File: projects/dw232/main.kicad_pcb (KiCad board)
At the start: 4 copper layers, 27 parts, among them P101 CONN_01X07, Q501 MMBT3904, Q502 MMBT3904, U501 LM741, U502 LM741, U503 2DW232

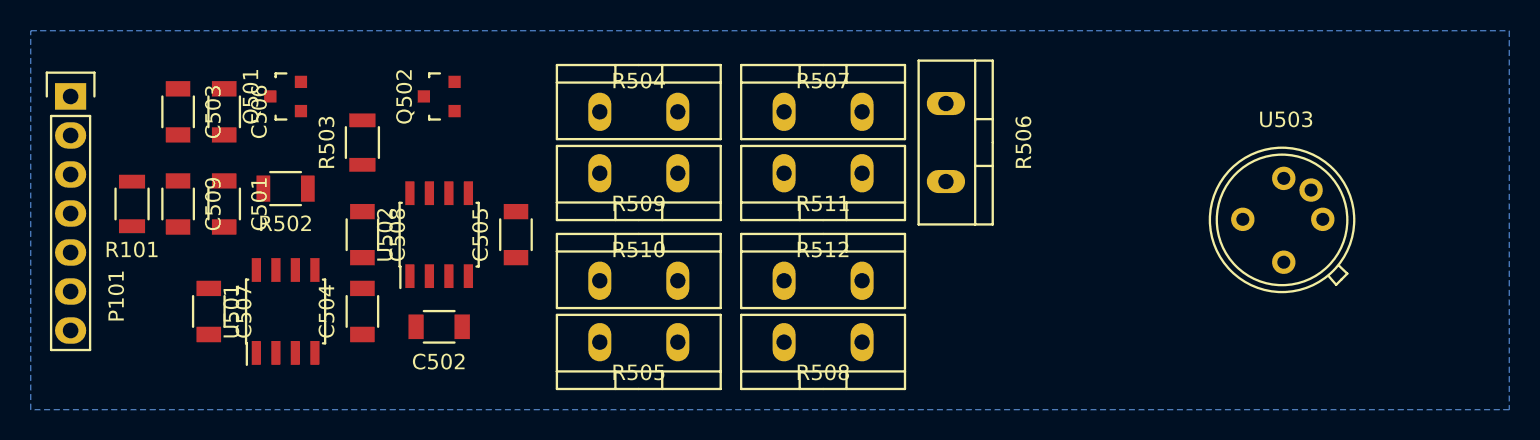
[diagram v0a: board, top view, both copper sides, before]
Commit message: remove old gerbers
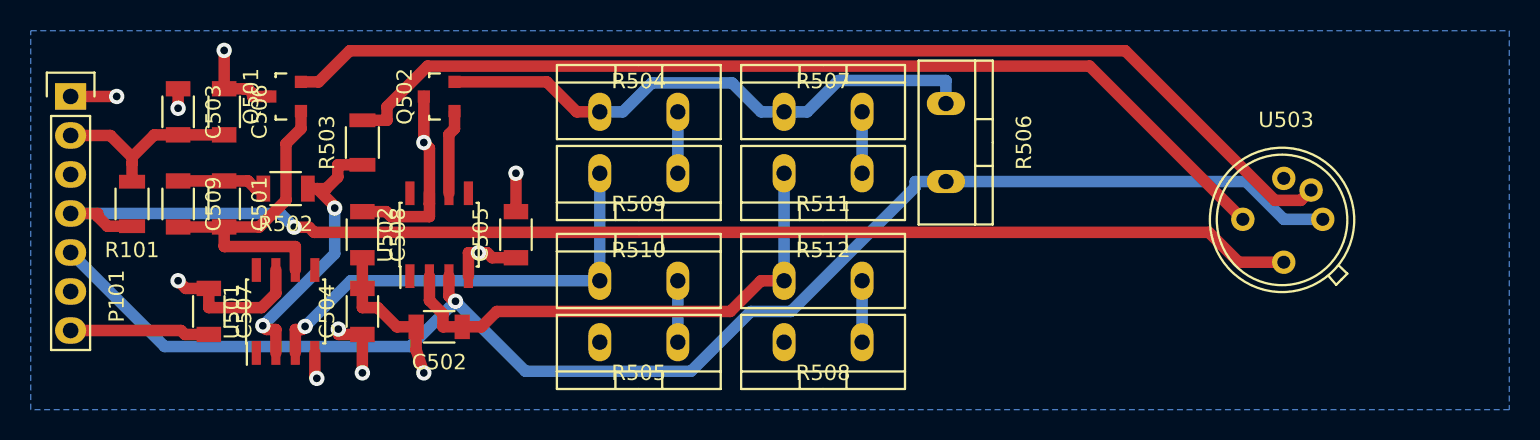
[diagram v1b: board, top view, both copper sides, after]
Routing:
- net REF: track 0.00 -> 95.4 mm, vias 0 -> 1
- net H-GND: track 0.00 -> 84.8 mm, vias 0 -> 1
- net Net-(Q501-Pad2): track 0.00 -> 70.9 mm
- net Net-(R503-Pad2): track 0.00 -> 63.4 mm
- net Net-(Q502-Pad2): track 0.00 -> 36.7 mm
- net AGND: track 0.00 -> 34.7 mm, vias 0 -> 2
- net Net-(C502-Pad1): track 0.00 -> 34.1 mm
- net +VE: track 0.00 -> 31.7 mm, vias 0 -> 4
- net Net-(R509-Pad2): track 0.00 -> 29.7 mm, vias 0 -> 1
- net Net-(C501-Pad2): track 0.00 -> 21.4 mm
- net Net-(R502-Pad1): track 0.00 -> 18.5 mm, vias 0 -> 2
- net -VE: track 0.00 -> 12.1 mm, vias 0 -> 5
- net Net-(C501-Pad1): track 0.00 -> 5.76 mm
- net Net-(Q502-Pad1): track 0.00 -> 5.50 mm
- net Net-(R508-Pad1): track 0.00 -> 4.00 mm
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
